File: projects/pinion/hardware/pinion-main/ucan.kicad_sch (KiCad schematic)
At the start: 0 parts

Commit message: [pinion] added all the sensors
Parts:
- added U10: TCAN1044VDRB, Texas_Instruments:Texas_DRB0008J_VSON-8-1EP_3x3mm_P0.65mm_EP1.65x2.4mm, symbol lib:TCAN1044VDRB
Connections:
- new net: U10.2 (GND), U10.9 (GND)
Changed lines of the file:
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@@
 	(generator_version "10.0")
 	(paper "A4")
+	(symbol
+		(lib_id "lib:TCAN1044VDRB")
+		(at 109.22 71.12 0)
+		(unit 1)
+		(body_style 1)
+		(exclude_from_sim no)
+		(in_bom yes)
+		(on_board yes)
+		(in_pos_files yes)
+		(dnp no)
+		(fields_autoplaced yes)
+		(property "Reference" "U10"
+			(at 111.3633 81.28 0)
+			(show_name no)
+			(do_not_autoplace no)
+			(effects
+				(font
+					(size 1.27 1.27)
+				)
+				(justify left)
+			)
+		)
+		(property "Value" "TCAN1044VDRB"
+			(at 111.3633 83.82 0)
+			(show_name no)
+			(do_not_autoplace no)
+			(effects
+				(font
+					(size 1.27 1.27)
+				)
+				(justify left)
+			)
+		)
+		(property "Footprint" "Texas_Instruments:Texas_DRB0008J_VSON-8-1EP_3x3mm_P0.65mm_EP1.65x2.4mm"
+			(at 109.22 71.12 0)
+			(hide yes)
+			(show_name no)
+			(do_not_autoplace no)
+			(effects
+				(font
+					(size 1.27 1.27)
+				)
+			)
+		)
+		(property "Datasheet" "https://www.ti.com/lit/ds/symlink/tcan1044-q1.pdf"
+			(at 109.22 71.12 0)
+			(hide yes)
+			(show_name no)
+			(do_not_autoplace no)
+			(effects
+				(font
+					(size 1.27 1.27)
+				)
+			)
+		)
+		(property "Description" "CAN FD transceiver with standby, 1.7V to 5.5V I/O supply (VIO), 8Mbps, VSON-8 3x3mm"
+			(at 109.22 71.12 0)
+			(hide yes)
+			(show_name no)
+			(do_not_autoplace no)
+			(effects
+				(font
+					(size 1.27 1.27)
+				)
+			)
+		)
+		(pin "2"
+		)
+		(pin "9"
+		)
+		(pin "5"
+		)
+		(pin "8"
+		)
+		(pin "7"
+		)
+		(pin "3"
+		)
+		(pin "6"
+		)
+		(pin "4"
+		)
+		(pin "1"
+		)
+		(instances
+			(project "pinion-main"
+				(path "/6c7907f5-5439-4f54-a5a2-0a7e85489635/e3d61feb-6226-49e9-91f2-6966c39438aa/be458081-d9d6-4cd1-9869-19004ca767b1"
+					(reference "U10")
+					(unit 1)
+				)
+			)
+		)
+	)
 )

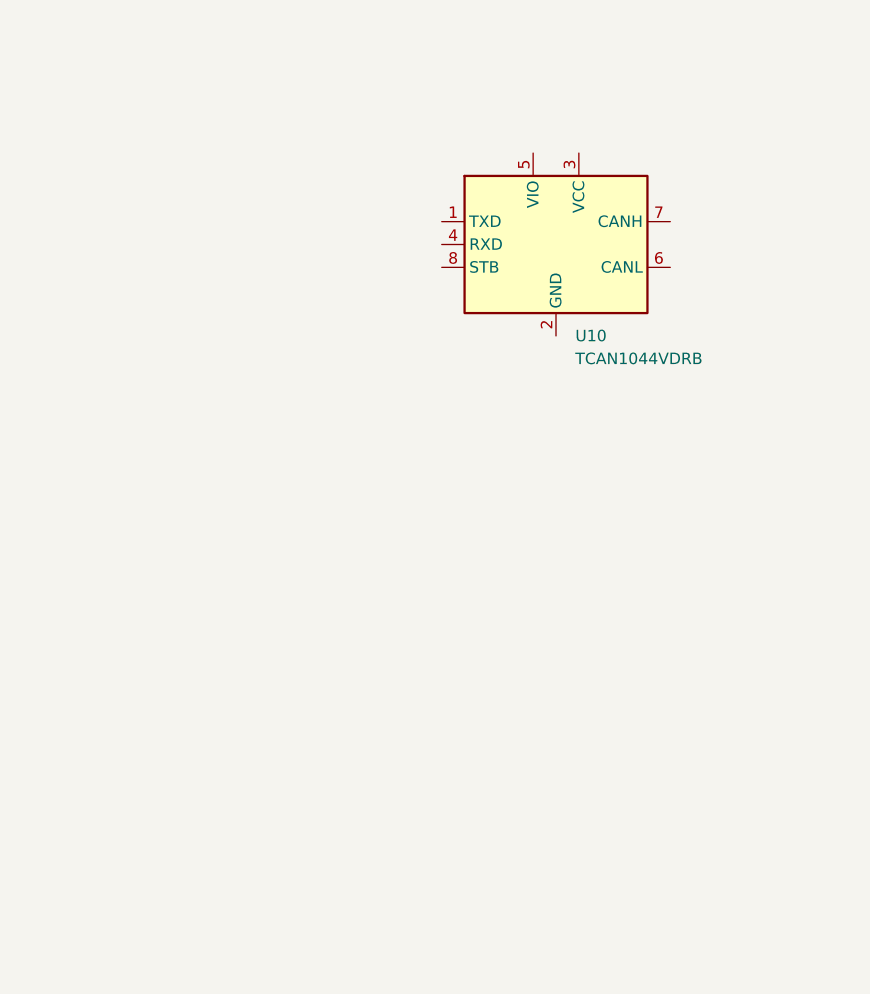
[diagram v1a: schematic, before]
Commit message: [pinion] fmu can transievers
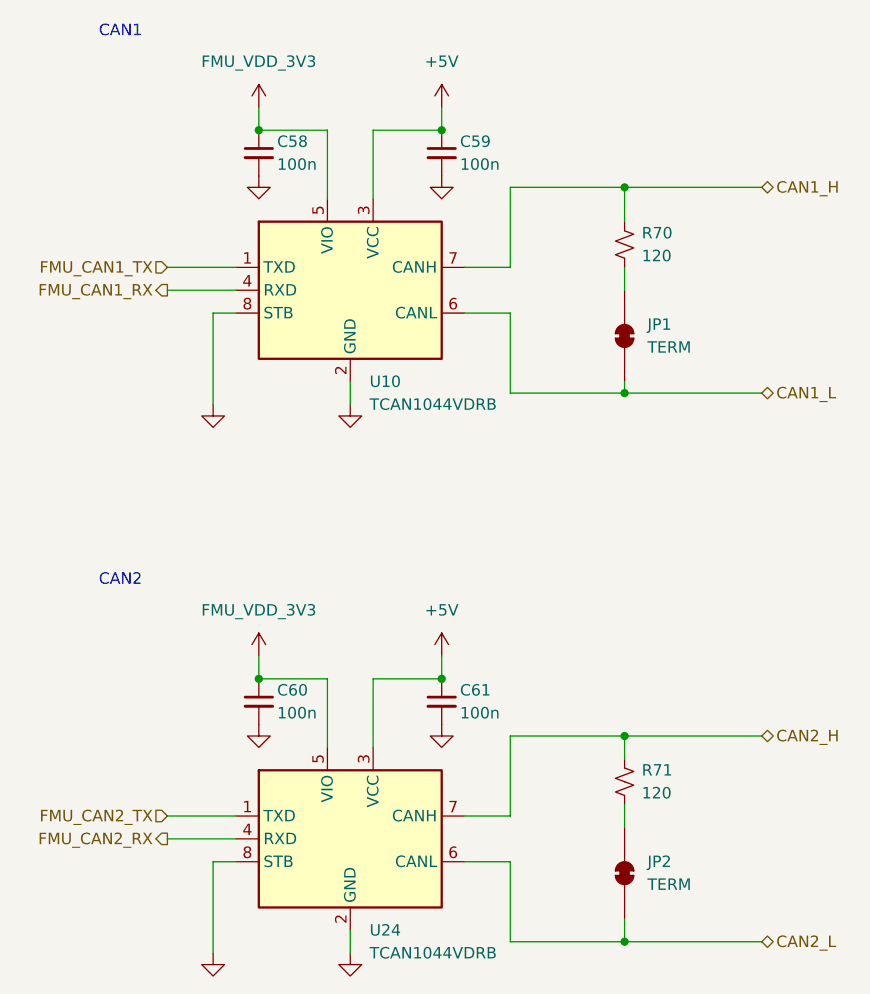
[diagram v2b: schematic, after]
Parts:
- added C58, C59, C60, C61: 100n, Capacitor_SMD:C_0402_1005Metric, symbol Device:C_Small
- added JP1, JP2: TERM, Jumper:SolderJumper-2_P1.3mm_Bridged_RoundedPad1.0x1.5mm, symbol Jumper:SolderJumper_2_Bridged
- added R70, R71: 120, Resistor_SMD:R_0603_1608Metric, symbol Device:R_Small_US
- added U24: TCAN1044VDRB, Texas_Instruments:Texas_DRB0008J_VSON-8-1EP_3x3mm_P0.65mm_EP1.65x2.4mm, symbol lib:TCAN1044VDRB
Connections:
- net FMU_CAN1_TX: now reaches U10.1 (TXD)
- net GND: now reaches U10.2 (GND), U10.9 (GND)
- net GND: now also U10.8 (STB), C58.2, C59.2, C60.2, C61.2, U24.2 (GND), U24.8 (STB), U24.9 (GND)
- net +5V: now reaches U10.3 (VCC)
- net +5V: now also C59.1, C61.1, U24.3 (VCC)
- net FMU_CAN1_RX: now reaches U10.4 (RXD)
- net FMU_VDD_3V3: now reaches U10.5 (VIO)
- net FMU_VDD_3V3: now also C58.1, C60.1, U24.5 (VIO)
- net CAN1_L: now reaches U10.6 (CANL)
- net CAN1_L: now also JP1.2 (B)
- net CAN1_H: now reaches U10.7 (CANH)
- net CAN1_H: now also R70.1
- new net: JP2.1 (A), R71.2
- new net: JP1.1 (A), R70.2
- new net CAN2_H: R71.1, U24.7 (CANH)
- new net CAN2_L: JP2.2 (B), U24.6 (CANL)
- new net FMU_CAN2_RX: U24.4 (RXD)
- new net FMU_CAN2_TX: U24.1 (TXD)
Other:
- note added: "CAN1"
- note added: "CAN2"
